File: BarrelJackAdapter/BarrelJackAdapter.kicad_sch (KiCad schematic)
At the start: 6 parts, among them J1 Barrel_Jack_Switch, J2 Conn_01x03, J4 Conn_01x03, U1 L7805

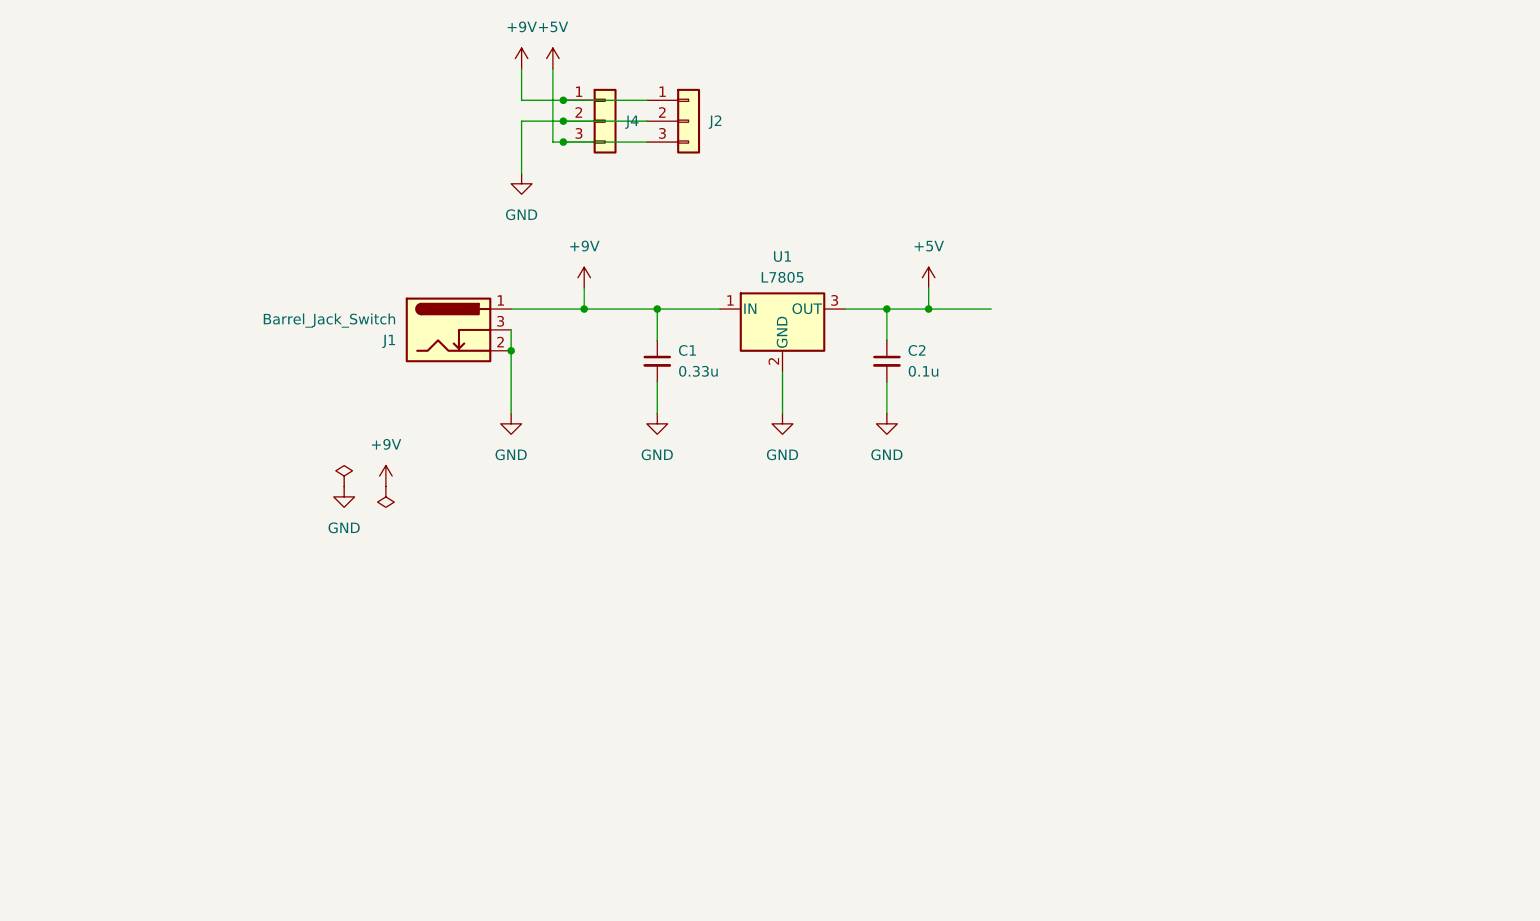
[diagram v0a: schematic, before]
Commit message: wip
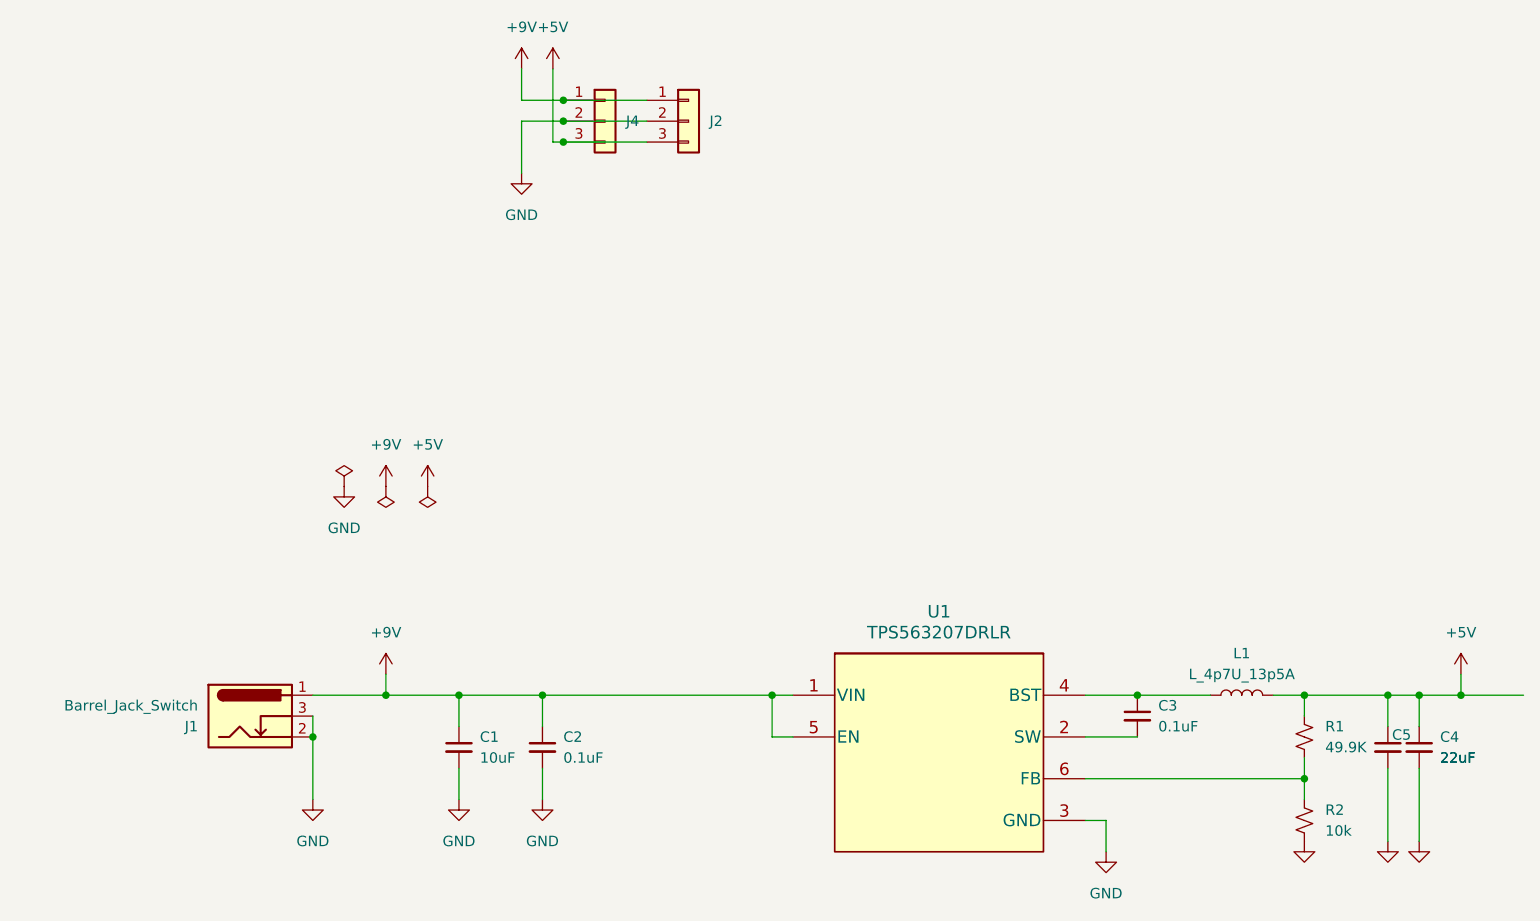
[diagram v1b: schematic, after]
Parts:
- removed C1: 0.33u, Capacitor_SMD:C_0603_1608Metric, symbol Device:C_Small
- removed C2: 0.1u, Capacitor_SMD:C_0603_1608Metric, symbol Device:C_Small
- removed U1: L7805, Package_TO_SOT_SMD:TO-263-2, symbol Regulator_Linear:L7805
- added C1: C_10U_805, Capacitor_SMD:C_0805_2012Metric, symbol StockedComponents:C_10U_805
- added C2, C3: C_P1U, Capacitor_SMD:C_0603_1608Metric, symbol StockedComponents:C_P1U
- added C4, C5: C_22U_1210, Capacitor_SMD:C_1210_3225Metric, symbol StockedComponents:C_22U_1210
- added L1: L_4p7U_13p5A, Inductor_SMD:L_Coilcraft_XxL4040, symbol StockedComponents:L_4p7U_13p5A
- added R1: R_49p9K, Resistor_SMD:R_0603_1608Metric, symbol StockedComponents:R_49p9K
- added R2: R_10K, Resistor_SMD:R_0603_1608Metric, symbol StockedComponents:R_10K
- added U1: TPS563207DRLR, Package_TO_SOT_SMD:SOT-563, symbol StockedComponents:TPS563207DRLR
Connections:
- net +5V: now also C4.1, C5.1, L1.2, R1.1
- net +9V: now also C1.1, C2.1, U1.1 (VIN), U1.5 (EN)
- net GND: now also C1.2, C2.2, C4.2, C5.2, R2.2, U1.3 (GND)
- new net: R1.2, R2.1, U1.6 (FB)
- new net: C3.1, L1.1, U1.4 (BST)
- new net: C3.2, U1.2 (SW)
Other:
- moved on the sheet: J1
